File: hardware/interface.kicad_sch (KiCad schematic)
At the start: 16 parts, among them J1 EXT_PWR, J2 GPIO, J3 I2C, J4 USB, J6 SPI, J8 SWD

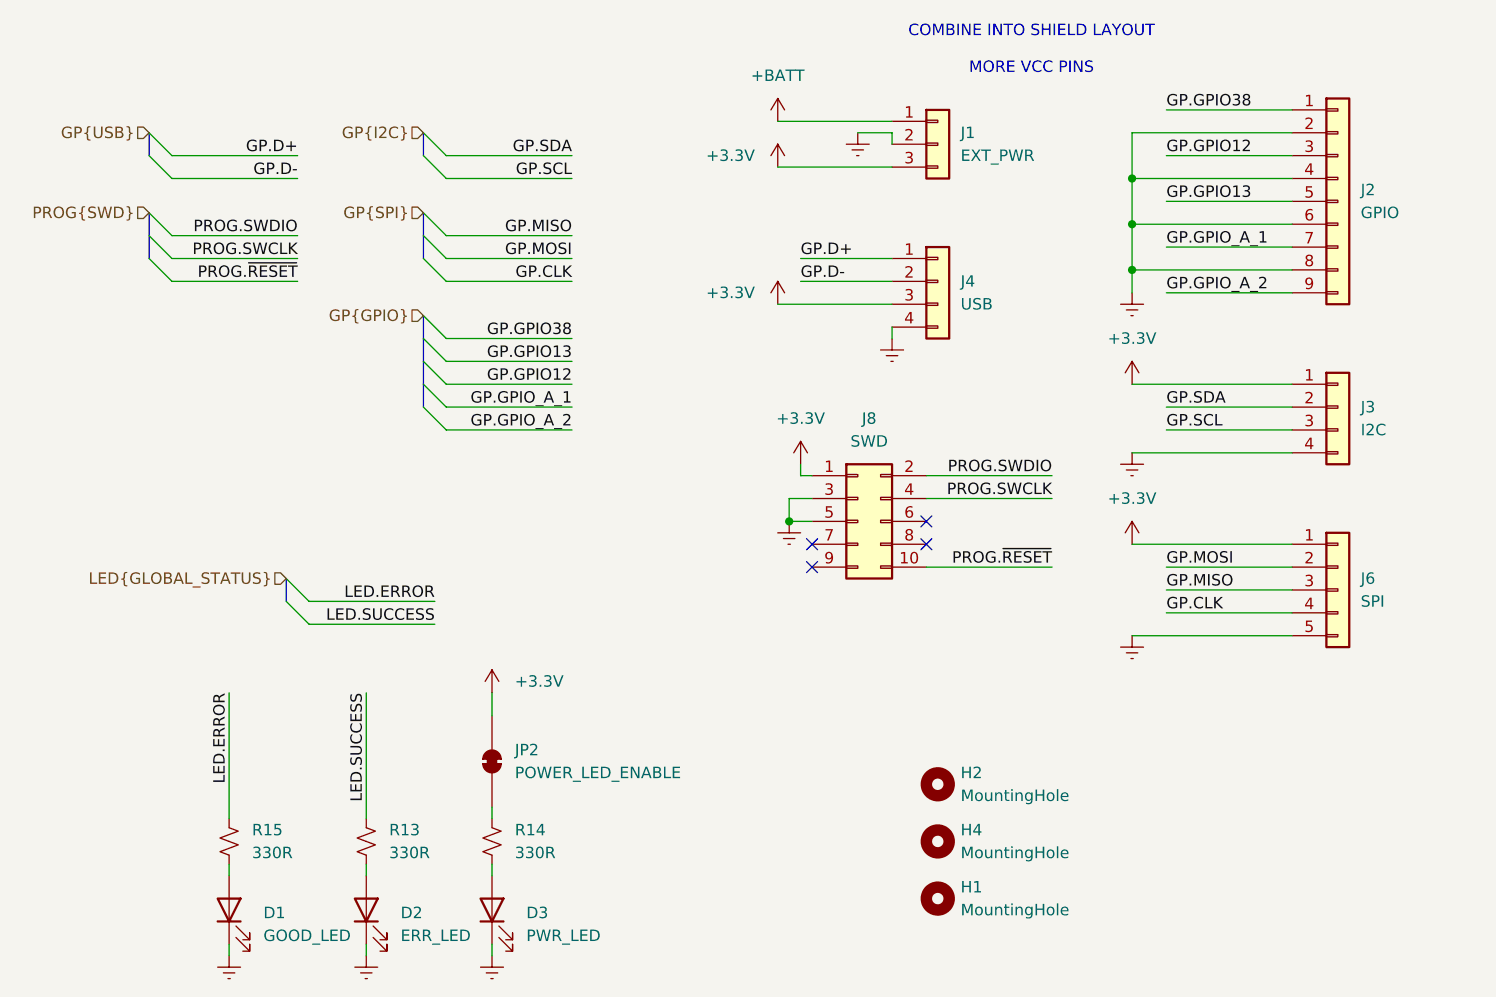
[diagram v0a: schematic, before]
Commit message: draft of gpio layout
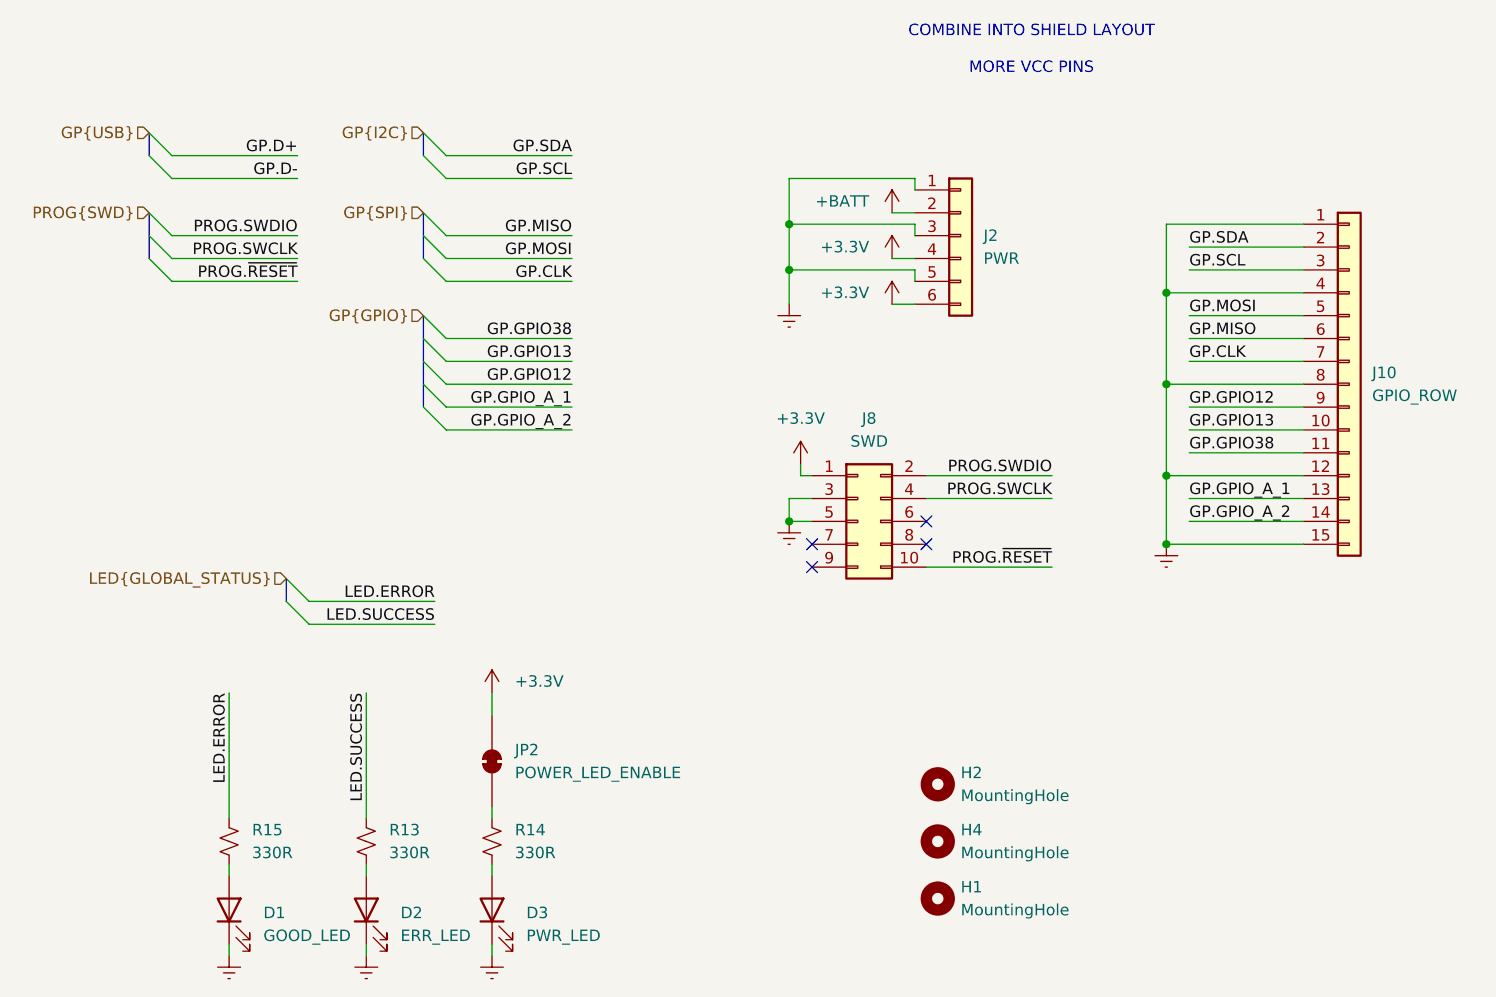
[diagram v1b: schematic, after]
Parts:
- removed J1: EXT_PWR, Connector_PinHeader_2.54mm:PinHeader_1x03_P2.54mm_Vertical, symbol Connector_Generic:Conn_01x03
- removed J2: GPIO, Connector_PinHeader_2.54mm:PinHeader_1x09_P2.54mm_Vertical, symbol Connector_Generic:Conn_01x09
- removed J3: I2C, Connector_PinHeader_2.54mm:PinHeader_1x04_P2.54mm_Vertical, symbol Connector_Generic:Conn_01x04
- removed J4: USB, Connector_PinHeader_2.54mm:PinHeader_1x04_P2.54mm_Vertical, symbol Connector_Generic:Conn_01x04
- removed J6: SPI, Connector_PinHeader_2.54mm:PinHeader_1x05_P2.54mm_Vertical, symbol Connector_Generic:Conn_01x05
- added J10: GPIO_ROW, Connector_PinHeader_2.54mm:PinHeader_1x15_P2.54mm_Vertical, symbol Connector_Generic:Conn_01x15
- added J2: PWR, Connector_PinHeader_2.54mm:PinHeader_1x06_P2.54mm_Vertical, symbol Connector_Generic:Conn_01x06
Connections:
- net +3.3V: now also J2.4 (Pin_4), J2.6 (Pin_6)
- net +BATT: now also J2.2 (Pin_2)
- net Earth: now also J10.1 (Pin_1), J10.12 (Pin_12), J10.15 (Pin_15), J10.4 (Pin_4), J10.8 (Pin_8), J2.1 (Pin_1), J2.3 (Pin_3), J2.5 (Pin_5)
- net GP.CLK: now also J10.7 (Pin_7)
- net GP.GPIO12: now also J10.9 (Pin_9)
- net GP.GPIO13: now also J10.10 (Pin_10)
- net GP.GPIO38: now also J10.11 (Pin_11)
- net GP.GPIO_A_1: now also J10.13 (Pin_13)
- net GP.GPIO_A_2: now also J10.14 (Pin_14)
- net GP.MISO: now also J10.6 (Pin_6)
- net GP.MOSI: now also J10.5 (Pin_5)
- net GP.SCL: now also J10.3 (Pin_3)
- net GP.SDA: now also J10.2 (Pin_2)

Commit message: net class shenanigans
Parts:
- D1, D2, D3, R13, R14, R15: KiLib_Generator (none) -> SMD_2terminal_chip_molded
- H1, H2, H4: KiLib_Generator (none) -> mounting_hardware/mounting_hole
- J10, J2: KiLib_Generator (none) -> connector/pin_header_socket
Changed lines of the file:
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@@
+			)
+		)
+		(property "KiLib_Generator" "SMD_2terminal_chip_molded"
+			(at 86.36 125.73 0)
+			(hide yes)
+			(show_name no)
+			(do_not_autoplace no)
+			(effects
+				(font
+					(size 1.27 1.27)
+				)
 			)
 		)
@@
 		)
 		(property "Mouser Price/Stock" ""
+			(at 115.57 125.73 0)
+			(hide yes)
+			(show_name no)
+			(do_not_autoplace no)
+			(effects
+				(font
+					(size 1.27 1.27)
+				)
+			)
+		)
+		(property "KiLib_Generator" "SMD_2terminal_chip_molded"
 			(at 115.57 125.73 0)
 			(hide yes)
@@
 			)
 		)
+		(property "KiLib_Generator" "SMD_2terminal_chip_molded"
+			(at 115.57 133.35 0)
+			(hide yes)
+			(show_name no)
+			(do_not_autoplace no)
+			(effects
+				(font
+					(size 1.27 1.27)
+				)
+			)
+		)
 		(pin "1"
 		)
@@
 		(property "Mouser Price/Stock" ""
 			(at 101.6 133.35 90)
+			(hide yes)
+			(show_name no)
+			(do_not_autoplace no)
+			(effects
+				(font
+					(size 1.27 1.27)
+				)
+			)
+		)
+		(property "KiLib_Generator" "SMD_2terminal_chip_molded"
+			(at 101.6 133.35 0)
 			(hide yes)
 			(show_name no)
@@
 			)
 		)
+		(property "KiLib_Generator" "mounting_hardware/mounting_hole"
+			(at 165.1 132.08 0)
+			(hide yes)
+			(show_name no)
+			(do_not_autoplace no)
+			(effects
+				(font
+					(size 1.27 1.27)
+				)
+			)
+		)
 		(instances
 			(project "Tiny4FSK"
@@
 			)
 		)
+		(property "KiLib_Generator" "mounting_hardware/mounting_hole"
+			(at 165.1 119.38 0)
+			(hide yes)
+			(show_name no)
+			(do_not_autoplace no)
+			(effects
+				(font
+					(size 1.27 1.27)
+				)
+			)
+		)
 		(instances
 			(project "Tiny4FSK"
@@
 		)
 		(property "Description" "Generic connector, single row, 01x15, script generated (kicad-library-utils/schlib/autogen/connector/)"
+			(at 210.82 74.93 0)
+			(hide yes)
+			(show_name no)
+			(do_not_autoplace no)
+			(effects
+				(font
+					(size 1.27 1.27)
+				)
+			)
+		)
+		(property "KiLib_Generator" "connector/pin_header_socket"
 			(at 210.82 74.93 0)
 			(hide yes)
@@
 			)
 		)
+		(property "KiLib_Generator" "SMD_2terminal_chip_molded"
+			(at 86.36 133.35 0)
+			(hide yes)
+			(show_name no)
+			(do_not_autoplace no)
+			(effects
+				(font
+					(size 1.27 1.27)
+				)
+			)
+		)
 		(pin "1"
 		)
@@
 		)
 		(property "Mouser Price/Stock" ""
+			(at 101.6 125.73 0)
+			(hide yes)
+			(show_name no)
+			(do_not_autoplace no)
+			(effects
+				(font
+					(size 1.27 1.27)
+				)
+			)
+		)
+		(property "KiLib_Generator" "SMD_2terminal_chip_molded"
 			(at 101.6 125.73 0)
 			(hide yes)
@@
 			)
 		)
+		(property "KiLib_Generator" "mounting_hardware/mounting_hole"
+			(at 165.1 125.73 0)
+			(hide yes)
+			(show_name no)
+			(do_not_autoplace no)
+			(effects
+				(font
+					(size 1.27 1.27)
+				)
+			)
+		)
 		(instances
 			(project "Tiny4FSK"
@@
 			(at 167.64 58.42 0)
 			(hide yes)
+			(show_name no)
+			(do_not_autoplace no)
+			(effects
+				(font
+					(size 1.27 1.27)
+				)
+			)
+		)
+		(property "KiLib_Generator" "connector/pin_header_socket"
+			(at 167.64 58.42 0)
+			(hide yes)
